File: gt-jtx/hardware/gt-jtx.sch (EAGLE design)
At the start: 6 parts, among them IC1 MEGA8-P

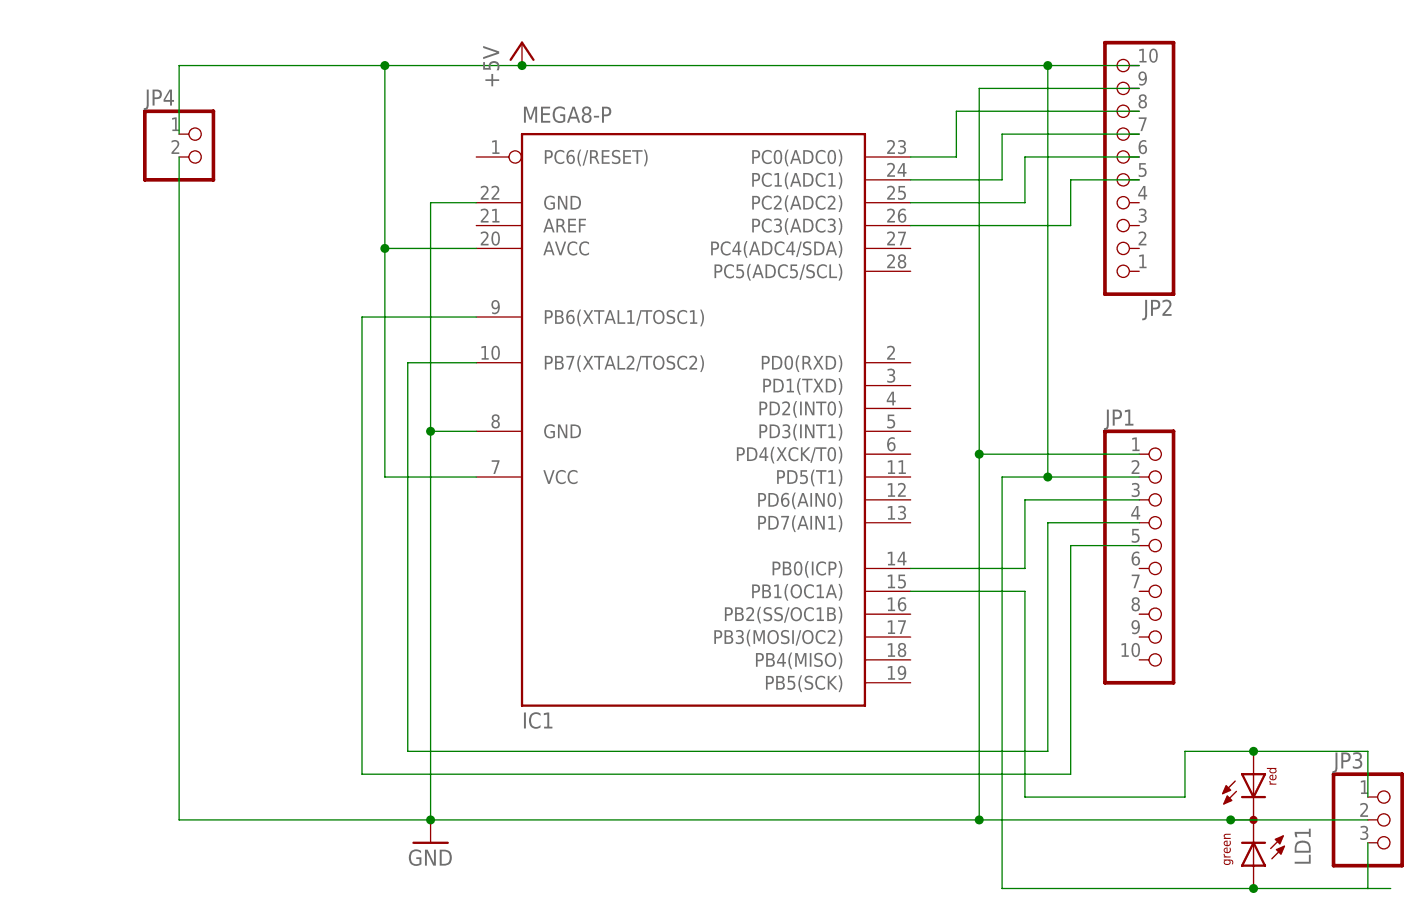
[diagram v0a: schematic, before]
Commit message: gt-jtx now has a board layout and a schematic.
git-svn-id: https://gt-jtx.googlecode.com/svn/trunk@15 79910f2a-facc-22ab-b1ea-80da55196309
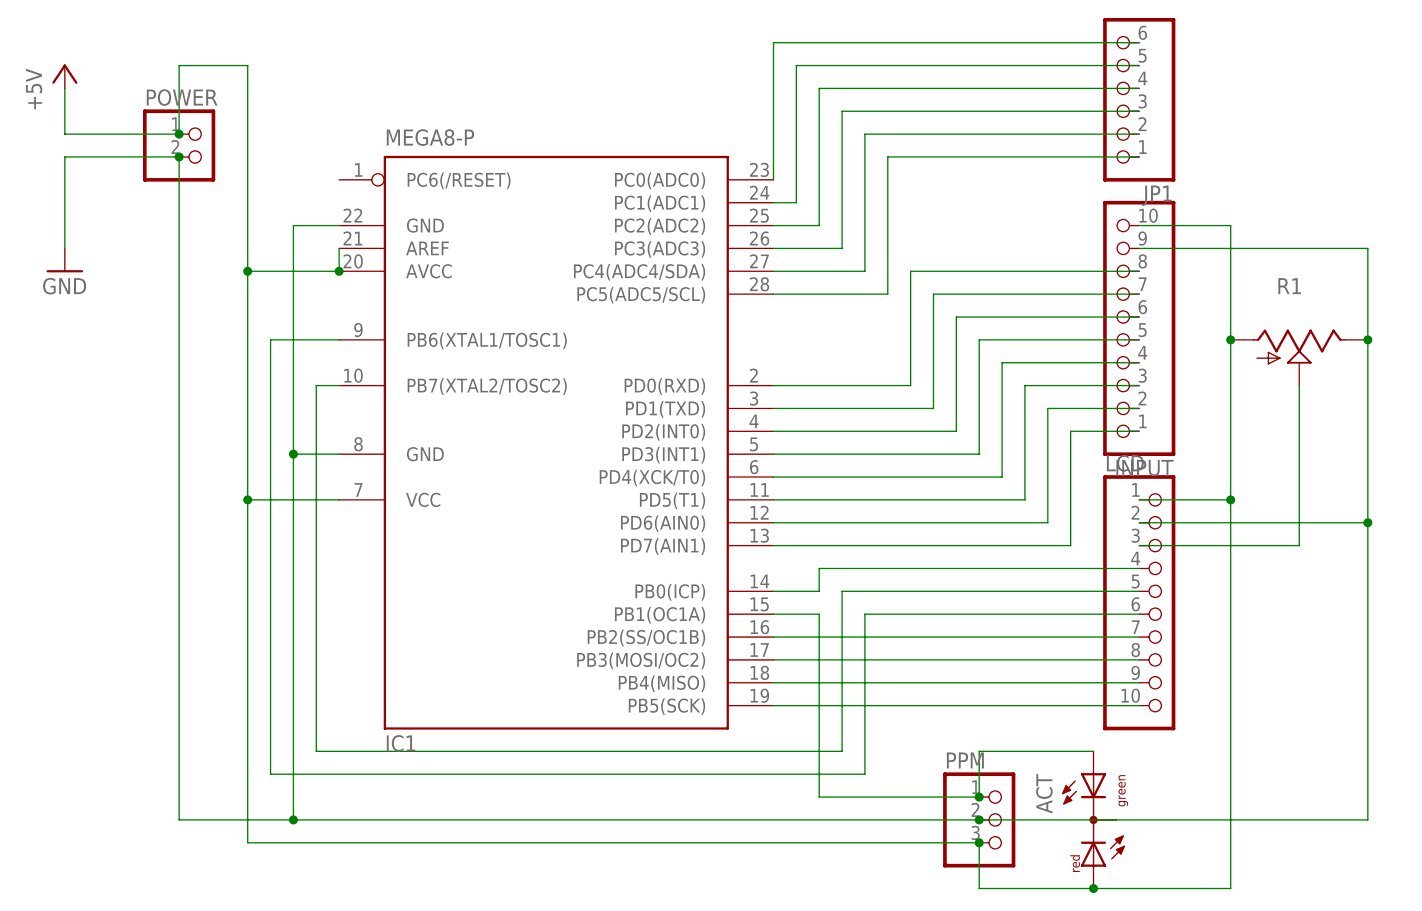
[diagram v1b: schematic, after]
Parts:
- removed JP2: (no value), pinhead:PINHD-1X10
- removed JP3: (no value), pinhead:PINHD-1X3
- removed LD1: (no value), led:DUOLED-RG-C
- added ACT: (no value), led:DUOLED-RG-C
- added INPUT, LCD: (no value), pinhead:PINHD-1X10
- added PPM: (no value), pinhead:PINHD-1X3
- added R1: (no value), pot:TRIM_US-CA6V
- JP1: device pinhead:PINHD-1X10 -> pinhead:PINHD-1X6
- renumbered JP4 to POWER
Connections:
- new net N$10: IC1.PC4(ADC4/SDA), JP1.2
- new net N$11: IC1.PC5(ADC5/SCL), JP1.1
- new net N$12: IC1.PB5(SCK), LCD.10
- new net N$13: IC1.PB4(MISO), LCD.9
- new net N$14: IC1.PB3(MOSI/OC2), LCD.8
- new net N$15: IC1.PB2(SS/OC1B), LCD.7
- new net N$16: ACT.AG, IC1.PB1(OC1A), PPM.1
- new net N$17: IC1.PD1(TXD), INPUT.7
- new net N$18: IC1.PD2(INT0), INPUT.6
- new net N$19: IC1.PD3(INT1), INPUT.5
- new net N$20: IC1.PD4(XCK/T0), INPUT.4
- new net N$21: IC1.PD5(T1), INPUT.3
- new net N$22: IC1.PD7(AIN1), INPUT.1
- new net N$23: IC1.PD6(AIN0), INPUT.2
- new net N$9: LCD.3, R1.S
- net +5V: now also ACT.AR, IC1.AREF, INPUT.10, LCD.1, PPM.3, R1.A; no longer JP1.2, JP2.10, JP3.3, LD1.AG
- net GND: now also ACT.C, INPUT.9, LCD.2, PPM.2, R1.E; no longer JP1.1, JP2.9, JP3.2, LD1.C
- net N$1: now also JP1.6; no longer JP2.8
- net N$2: now also JP1.5; no longer JP2.7
- net N$3: now also JP1.4; no longer JP2.6
- net N$4: now also JP1.3; no longer JP2.5
- net N$5: now also LCD.4; no longer JP1.3
- net N$6: now also LCD.5; no longer JP1.4
- net N$7: now also LCD.6; no longer JP1.5
- net N$8: now also IC1.PD0(RXD), INPUT.8; no longer IC1.PB1(OC1A), JP3.1, LD1.AR
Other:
- moved on the sheet: IC1
